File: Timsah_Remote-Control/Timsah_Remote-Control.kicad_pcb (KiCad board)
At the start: 2 copper layers, 160 x 100 mm, 45 parts, among them J1 Güç Girişi, J2 ICSP, J3 Klemens, SW1 Oto Depth, SW10 Backward, SW2 Lights, SW3 Up, SW4 Down, SW5 Power, SW6 Turn Back, SW7 Forward, SW8 Right, SW9 Left, U1 MAX485E, U2 LM7805_TO220, U3 PIC18F45K22-IP, U4 Joystick A, U5 Joystick B

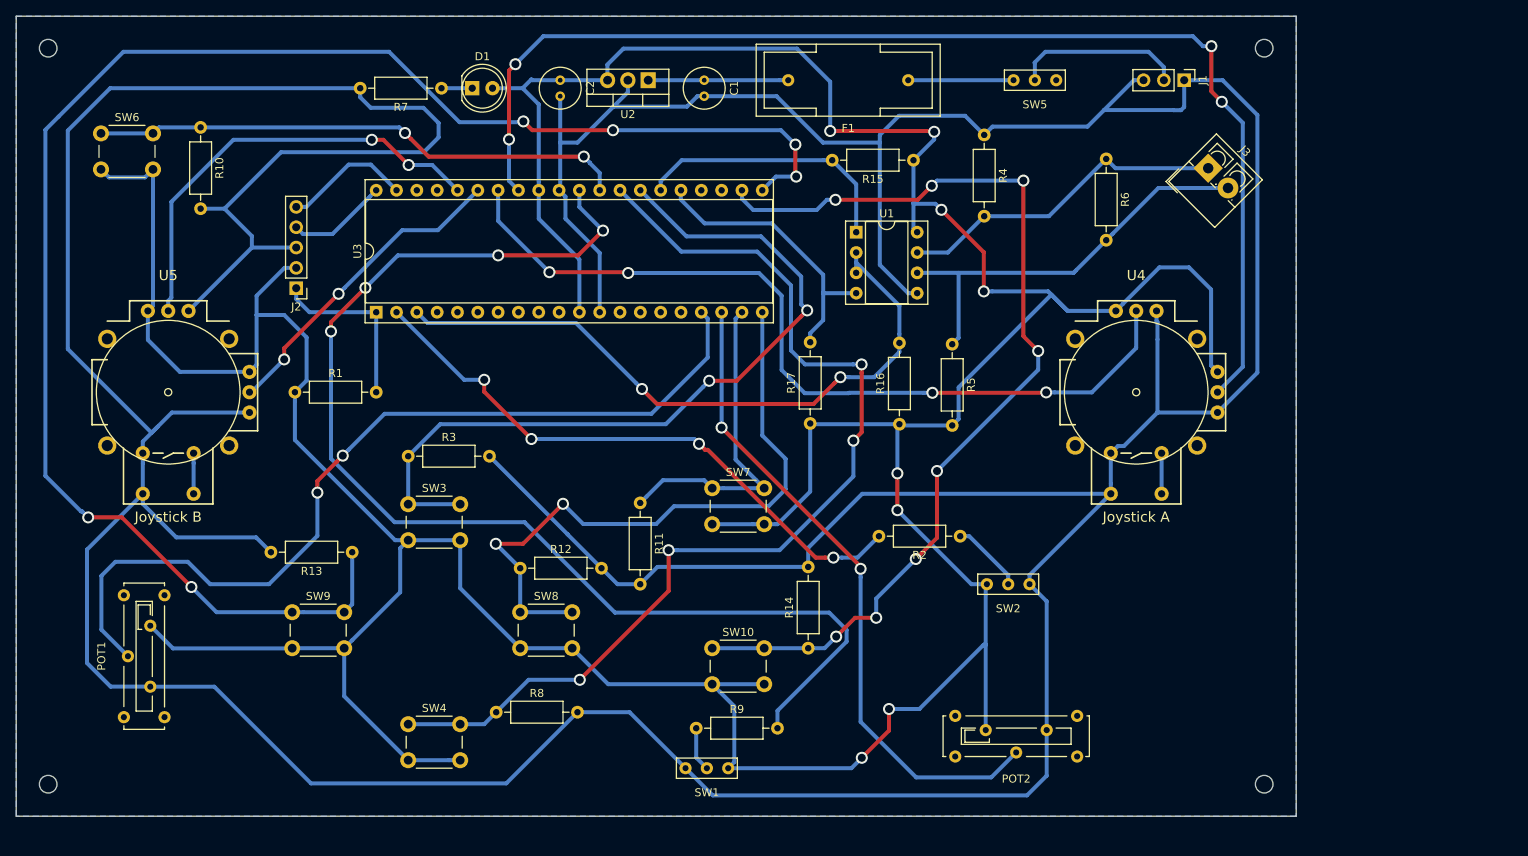
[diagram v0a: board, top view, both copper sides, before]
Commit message: Remote control board recreated.
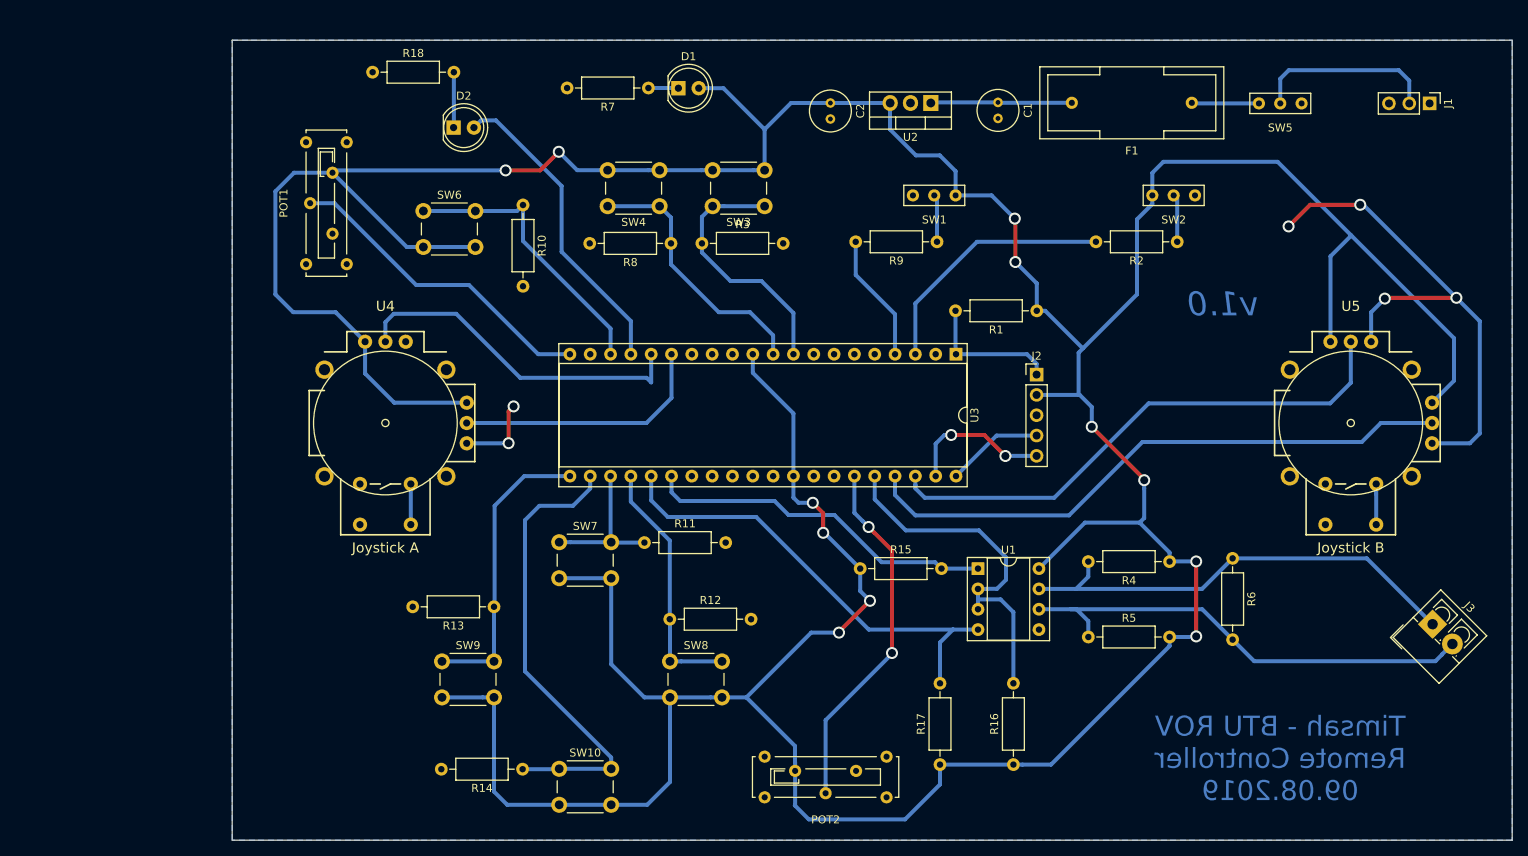
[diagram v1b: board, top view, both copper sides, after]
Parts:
- removed REF** (x4): MountingHole_2.2mm_M2, MountingHole:MountingHole_2.2mm_M2
- added D2: LED, LED_THT:LED_D5.0mm, F.Cu at (99.7, 58.9)
- added R18: 1k, Resistor_THT:R_Axial_DIN0207_L6.3mm_D2.5mm_P10.16mm_Horizontal, F.Cu at (89.5, 52.0)
- moved U5 147.9 mm to (211.8, 95.8)
- moved U4 93.9 mm to (91.2, 95.8)
- moved R1 93.3 mm to (172.6, 81.8), turned to 180 degrees
- moved J2 93.2 mm to (172.6, 89.8), turned to 0 degrees
- moved SW1 77.0 mm to (159.8, 67.4)
- moved U3 72.7 mm to (162.5, 87.2), turned to 270 degrees
- moved SW4 72.0 mm to (125.4, 68.8), turned to 180 degrees
- moved R9 67.8 mm to (160.1, 73.2), turned to 180 degrees
- moved J3 63.5 mm to (222.1, 121.0)
- moved R8 62.5 mm to (126.8, 73.4), turned to 180 degrees
- moved POT1 61.0 mm to (83.8, 68.4)
- moved R4 58.2 mm to (189.2, 113.2), turned to 180 degrees
- moved SW3 58.1 mm to (138.6, 68.8), turned to 180 degrees
- moved SW2 52.8 mm to (189.7, 67.4)
- moved R6 52.4 mm to (197.1, 112.8)
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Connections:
- R4 pad 1: GND -> +5V
- U3 pad 10: Net-(U3-Pad10) -> Down
- U3 pad 15: Net-(U3-Pad15) -> VRX-A
- U3 pad 16: Net-(U3-Pad16) -> VRY-A
- U3 pad 17: SERVO_Cam -> LED
- U3 pad 18: SERVO_Grip -> TURN_BACK
- U3 pad 19: Forward -> Net-(U3-Pad19)
- U3 pad 2: SW -> Net-(U3-Pad2)
- U3 pad 20: Right -> SERVO_Cam
- U3 pad 23: Net-(U3-Pad23) -> Forward
- U3 pad 24: Net-(U3-Pad24) -> Right
- U3 pad 27: Up -> Net-(U3-Pad27)
- U3 pad 28: Down -> Net-(U3-Pad28)
- U3 pad 29: TURN_BACK -> Net-(U3-Pad29)
- U3 pad 3: ENABLE -> SW
- U3 pad 30: OTO_DEPTH -> Net-(U3-Pad30)
- U3 pad 33: VRX-A -> Net-(U3-Pad33)
- U3 pad 34: VRY-A -> Net-(U3-Pad34)
- U3 pad 35: VRX-B -> SERVO_Grip
- U3 pad 36: VRY-B -> ENABLE
- U3 pad 37: Net-(U3-Pad37) -> VRX-B
- U3 pad 38: Net-(U3-Pad38) -> VRY-B
- U3 pad 4: Net-(U3-Pad4) -> OTO_DEPTH
- U3 pad 9: Net-(U3-Pad9) -> Up
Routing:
- net GND: track 718.7 -> 76.7 mm, vias 0 -> 6
- net Left: track 207.2 -> 36.9 mm, vias 6 -> 0
- net OTO_DEPTH: track 151.2 -> 16.1 mm, vias 4 -> 0
- net VRX-A: track 151.7 -> 32.4 mm, vias 4 -> 0
- net Down: track 129.9 -> 33.2 mm, vias 4 -> 0
- net SERVO_Cam: track 110.8 -> 40.3 mm, vias 2 -> 0
- net Up: track 99.0 -> 32.6 mm, vias 2 -> 0
- net Backward: track 124.2 -> 58.0 mm, vias 8 -> 0
- net VRY-A: track 104.9 -> 43.2 mm, vias 4 -> 0
- net Right: track 80.8 -> 31.7 mm, vias 2 -> 0
- net +5V: track 552.9 -> 596.0 mm, vias 8 -> 12
- net SW: track 75.0 -> 32.1 mm, vias 4 -> 0
- net LED: track 0.00 -> 39.3 mm
- net ENABLE: track 83.7 -> 45.6 mm, vias 2 -> 0
- net SERVO_Grip: track 82.0 -> 45.0 mm
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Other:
- board text added: "Timsah - BTU ROV Remote Controller 09.08.2019"
- board text added: "v1.0"
